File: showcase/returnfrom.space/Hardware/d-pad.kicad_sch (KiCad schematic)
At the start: 8 parts, among them SW19 SW_SPST, SW20 SW_SPST, SW21 SW_SPST, SW22 SW_SPST

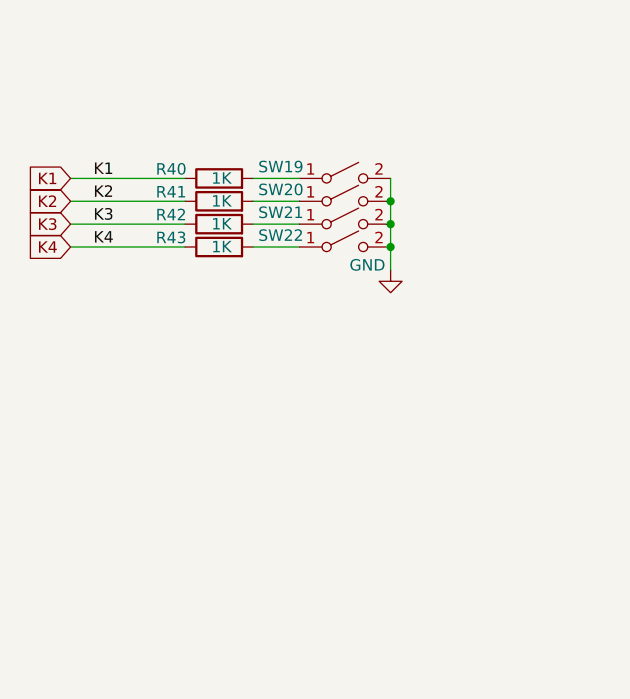
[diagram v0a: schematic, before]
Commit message: board almost done
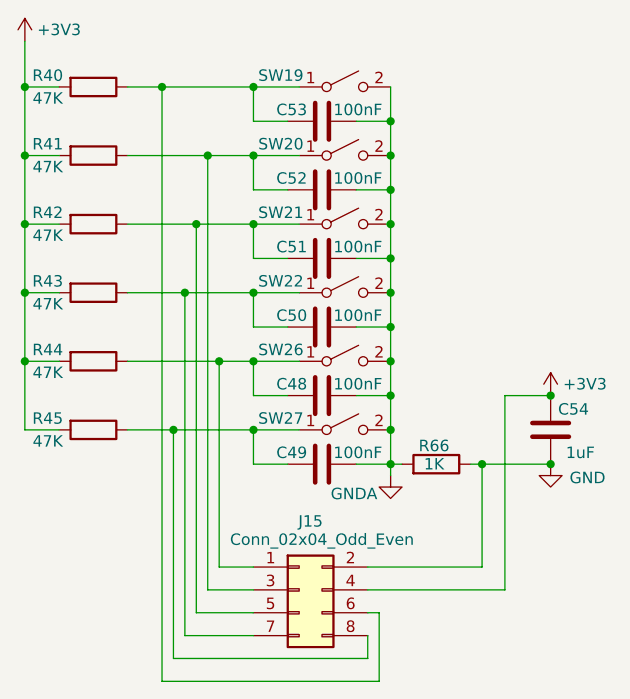
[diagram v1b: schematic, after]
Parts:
- added C48, C49, C50, C51, C52, C53: 100nF, Capacitor_SMD:C_0402_1005Metric, symbol Device:C
- added C54: 1uF, Capacitor_SMD:C_0402_1005Metric, symbol Device:C
- added J15: Conn_02x04_Odd_Even, Connector_PinSocket_2.54mm:PinSocket_2x04_P2.54mm_Vertical, symbol Connector_Generic:Conn_02x04_Odd_Even
- added R44, R45: 47K, Resistor_SMD:R_0402_1005Metric, symbol Device:R
- added R66: 1K, Resistor_SMD:R_0402_1005Metric, symbol Device:R
- added SW26, SW27: SW_SPST, Button_Switch_SMD:SW_SPST_TL3305C, symbol Switch:SW_SPST
- R40, R41, R42, R43: value 1K -> 47K
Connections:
- net K1 is gone; now on an unnamed net: R40.1
- net K2 is gone; now on an unnamed net: R41.1
- net K3 is gone; now on an unnamed net: R42.1
- net K4 is gone; now on an unnamed net: R43.1
- net GND: now also C54.1, J15.2 (Pin_2), R66.1; no longer SW19.2 (B), SW20.2 (B), SW21.2 (B), SW22.2 (B)
- net at SW20.1 (A): now also C52.2, J15.3 (Pin_3); no longer R41.2
- net at SW21.1 (A): now also C51.2, J15.5 (Pin_5); no longer R42.2
- net at SW22.1 (A): now also C50.2, J15.7 (Pin_7); no longer R43.2
- net at SW19.1 (A): now also C53.2, J15.6 (Pin_6); no longer R40.2
- new net: C48.2, J15.1 (Pin_1), R44.1, SW26.1 (A)
- new net: C49.2, J15.8 (Pin_8), R45.1, SW27.1 (A)
- new net +3V3: C54.2, J15.4 (Pin_4), R40.2, R41.2, R42.2, R43.2, R44.2, R45.2
- new net GNDA: C48.1, C49.1, C50.1, C51.1, C52.1, C53.1, R66.2, SW19.2 (B), SW20.2 (B), SW21.2 (B), SW22.2 (B), SW26.2 (B), SW27.2 (B)
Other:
- moved on the sheet: SW19, SW20, SW22
